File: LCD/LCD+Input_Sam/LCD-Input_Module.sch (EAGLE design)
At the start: 23 parts

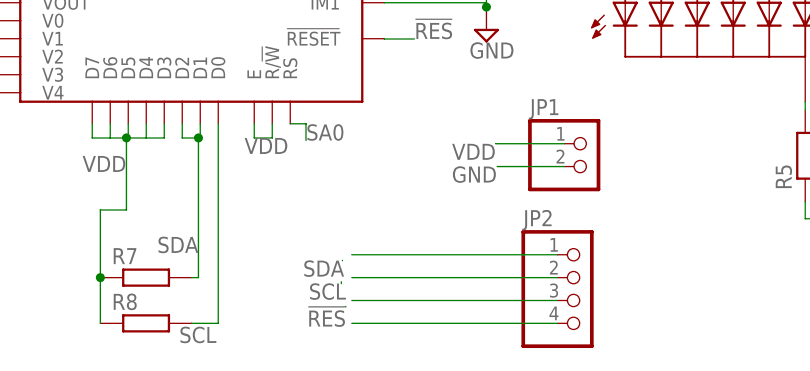
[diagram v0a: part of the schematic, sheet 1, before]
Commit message: LCD PCB final touches
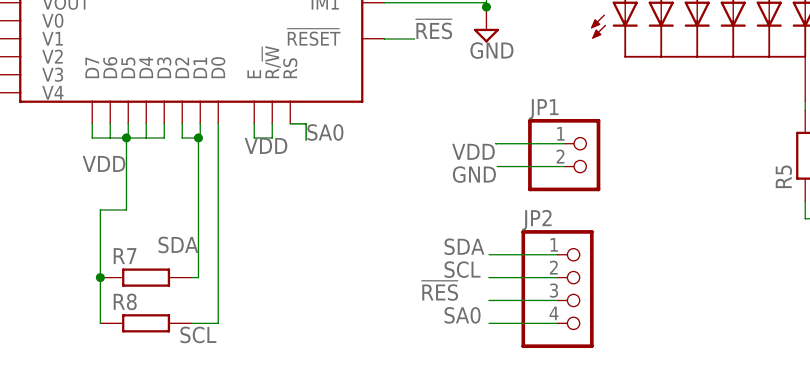
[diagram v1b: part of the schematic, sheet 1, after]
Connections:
- removed net N$1: JP2.3
- removed net N$2: JP2.2
- removed net N$3: JP2.1
- removed net N$8: JP2.4
- net !RES: now also JP2.3
- net SA0: now also JP2.4
- net SCL: now also JP2.2
- net SDA: now also JP2.1
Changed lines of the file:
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@@
 <grid distance="0.1" unitdist="inch" unit="inch" style="lines" multiple="1" display="no" altdistance="0.01" altunitdist="inch" altunit="inch"/>
 <layers>
-<layer number="1" name="Top" color="4" fill="1" visible="no" active="no"/>
-<layer number="16" name="Bottom" color="1" fill="1" visible="no" active="no"/>
-<layer number="17" name="Pads" color="2" fill="1" visible="no" active="no"/>
-<layer number="18" name="Vias" color="2" fill="1" visible="no" active="no"/>
-<layer number="19" name="Unrouted" color="6" fill="1" visible="no" active="no"/>
-<layer number="20" name="Dimension" color="24" fill="1" visible="no" active="no"/>
-<layer number="21" name="tPlace" color="7" fill="1" visible="no" active="no"/>
-<layer number="22" name="bPlace" color="7" fill="1" visible="no" active="no"/>
-<layer number="23" name="tOrigins" color="15" fill="1" visible="no" active="no"/>
-<layer number="24" name="bOrigins" color="15" fill="1" visible="no" active="no"/>
-<layer number="25" name="tNames" color="7" fill="1" visible="no" active="no"/>
-<layer number="26" name="bNames" color="7" fill="1" visible="no" active="no"/>
-<layer number="27" name="tValues" color="7" fill="1" visible="no" active="no"/>
-<layer number="28" name="bValues" color="7" fill="1" visible="no" active="no"/>
+<layer number="1" name="Top" color="4" fill="1" visible="yes" active="no"/>
+<layer number="16" name="Bottom" color="1" fill="1" visible="yes" active="no"/>
+<layer number="17" name="Pads" color="2" fill="1" visible="yes" active="no"/>
+<layer number="18" name="Vias" color="2" fill="1" visible="yes" active="no"/>
+<layer number="19" name="Unrouted" color="6" fill="1" visible="yes" active="no"/>
+<layer number="20" name="Dimension" color="24" fill="1" visible="yes" active="no"/>
+<layer number="21" name="tPlace" color="7" fill="1" visible="yes" active="no"/>
+<layer number="22" name="bPlace" color="7" fill="1" visible="yes" active="no"/>
+<layer number="23" name="tOrigins" color="15" fill="1" visible="yes" active="no"/>
+<layer number="24" name="bOrigins" color="15" fill="1" visible="yes" active="no"/>
+<layer number="25" name="tNames" color="7" fill="1" visible="yes" active="no"/>
+<layer number="26" name="bNames" color="7" fill="1" visible="yes" active="no"/>
+<layer number="27" name="tValues" color="7" fill="1" visible="yes" active="no"/>
+<layer number="28" name="bValues" color="7" fill="1" visible="yes" active="no"/>
 <layer number="29" name="tStop" color="7" fill="3" visible="no" active="no"/>
 <layer number="30" name="bStop" color="7" fill="6" visible="no" active="no"/>
@@
 <layer number="35" name="tGlue" color="7" fill="4" visible="no" active="no"/>
 <layer number="36" name="bGlue" color="7" fill="5" visible="no" active="no"/>
-<layer number="37" name="tTest" color="7" fill="1" visible="no" active="no"/>
-<layer number="38" name="bTest" color="7" fill="1" visible="no" active="no"/>
+<layer number="37" name="tTest" color="7" fill="1" visible="yes" active="no"/>
+<layer number="38" name="bTest" color="7" fill="1" visible="yes" active="no"/>
 <layer number="39" name="tKeepout" color="4" fill="11" visible="no" active="no"/>
 <layer number="40" name="bKeepout" color="1" fill="11" visible="no" active="no"/>
@@
 <layer number="44" name="Drills" color="7" fill="1" visible="no" active="no"/>
 <layer number="45" name="Holes" color="7" fill="1" visible="no" active="no"/>
-<layer number="46" name="Milling" color="3" fill="1" visible="no" active="no"/>
-<layer number="47" name="Measures" color="7" fill="1" visible="no" active="no"/>
-<layer number="48" name="Document" color="7" fill="1" visible="no" active="no"/>
-<layer number="49" name="Reference" color="7" fill="1" visible="no" active="no"/>
-<layer number="51" name="tDocu" color="7" fill="1" visible="no" active="no"/>
-<layer number="52" name="bDocu" color="7" fill="1" visible="no" active="no"/>
+<layer number="46" name="Milling" color="3" fill="1" visible="yes" active="no"/>
+<layer number="47" name="Measures" color="7" fill="1" visible="yes" active="no"/>
+<layer number="48" name="Document" color="7" fill="1" visible="yes" active="no"/>
+<layer number="49" name="Reference" color="7" fill="1" visible="yes" active="no"/>
+<layer number="51" name="tDocu" color="7" fill="1" visible="yes" active="no"/>
+<layer number="52" name="bDocu" color="7" fill="1" visible="yes" active="no"/>
 <layer number="88" name="SimResults" color="9" fill="1" visible="yes" active="yes"/>
 <layer number="89" name="SimProbes" color="9" fill="1" visible="yes" active="yes"/>
@@
 <net name="SDA" class="0">
 <segment>
-<wire x1="65" y1="32.36" x2="65" y2="32.395" width="0.1524" layer="91"/>
-<label x="65.2" y="32.37" size="1.778" layer="95" rot="R180"/>
-</segment>
-<segment>
 <pinref part="U$1" gate="G$1" pin="D2"/>
 <wire x1="47.2" y1="47.565" x2="47.2" y2="46" width="0.1524" layer="91"/>
@@
 <wire x1="49" y1="46" x2="49" y2="30.48" width="0.1524" layer="91"/>
 <wire x1="49" y1="30.48" x2="48.26" y2="30.48" width="0.1524" layer="91"/>
+</segment>
+<segment>
+<pinref part="JP2" gate="A" pin="1"/>
+<wire x1="88.9" y1="33.02" x2="81.28" y2="33.02" width="0.1524" layer="91"/>
+<label x="76.2" y="33.02" size="1.778" layer="95"/>
 </segment>
 </net>
@@
 <net name="!RES" class="0">
 <segment>
-<wire x1="65.375" y1="27.28" x2="65.375" y2="27.22" width="0.1524" layer="91"/>
-<label x="65.4" y="26.82" size="1.778" layer="95" rot="R180"/>
-</segment>
-<segment>
 <pinref part="U$1" gate="G$1" pin="!RESET"/>
 <wire x1="69.66" y1="57.025" x2="69.66" y2="57" width="0.1524" layer="91"/>
@@
 <label x="73" y="57" size="1.778" layer="95"/>
 </segment>
+<segment>
+<pinref part="JP2" gate="A" pin="3"/>
+<wire x1="81.28" y1="27.94" x2="88.9" y2="27.94" width="0.1524" layer="91"/>
+<label x="73.66" y="27.94" size="1.778" layer="95"/>
+</segment>
 </net>
 <net name="SCL" class="0">
-<segment>
-<wire x1="64.875" y1="29.82" x2="64.875" y2="30.02" width="0.1524" layer="91"/>
-<label x="65.4" y="29.82" size="1.778" layer="95" rot="R180"/>
-</segment>
 <segment>
 <pinref part="R8" gate="G$1" pin="2"/>
@@
 <wire x1="51.2" y1="25.4" x2="51.2" y2="47.565" width="0.1524" layer="91"/>
 <label x="51" y="25" size="1.778" layer="95" rot="R180"/>
+</segment>
+<segment>
+<pinref part="JP2" gate="A" pin="2"/>
+<wire x1="81.28" y1="30.48" x2="88.9" y2="30.48" width="0.1524" layer="91"/>
+<label x="76.2" y="30.48" size="1.778" layer="95"/>
 </segment>
 </net>
@@
 <label x="60.96" y="45.72" size="1.778" layer="95"/>
 </segment>
-</net>
-<net name="N$1" class="0">
-<segment>
-<pinref part="JP2" gate="A" pin="3"/>
-<wire x1="66.04" y1="27.94" x2="88.9" y2="27.94" width="0.1524" layer="91"/>
-</segment>
-</net>
-<net name="N$2" class="0">
-<segment>
-<pinref part="JP2" gate="A" pin="2"/>
-<wire x1="66.04" y1="30.48" x2="88.9" y2="30.48" width="0.1524" layer="91"/>
-</segment>
-</net>
-<net name="N$3" class="0">
-<segment>
-<pinref part="JP2" gate="A" pin="1"/>
-<wire x1="66.04" y1="33.02" x2="88.9" y2="33.02" width="0.1524" layer="91"/>
-</segment>
-</net>
-<net name="N$8" class="0">
 <segment>
 <pinref part="JP2" gate="A" pin="4"/>
-<wire x1="88.9" y1="25.4" x2="66.04" y2="25.4" width="0.1524" layer="91"/>
-</segment>
-</net>
+<wire x1="88.9" y1="25.4" x2="81.28" y2="25.4" width="0.1524" layer="91"/>
+<label x="76.2" y="25.4" size="1.778" layer="95"/>
+</segment>
+</net>
